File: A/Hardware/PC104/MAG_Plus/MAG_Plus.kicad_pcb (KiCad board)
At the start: 2 copper layers, 96 x 89.9 mm, 106 parts, among them J1 RPi_GPIO, J2 U.FL-R-SMT(01), J3 U.FL-R-SMT(01), J4 U.FL-R-SMT(01), J5 U.FL-R-SMT(01), J6 Conn_01x12_Male, J7 Conn_01x04_Male, J8 Conn_01x04_Male, J9 Conn_01x06_Male, SW1 SW_Push, U1 Payload, U10 QPQ1906SR, U11 ISO7341C, U12 PIC16F1847-I_SO, U13 LP38693MP-3.3, U14 LP38693MP-3.3, U15 LP38693MP-5.0, U16 LP38693MP-3.3, U2 ISO1540, U3 ISO7341C, U4 AD8302, U5 AD8302, U6 AD7904BRUZ-REEL7, U7 QPQ1906SR, U8 QPQ1906SR, U9 QPQ1906SR

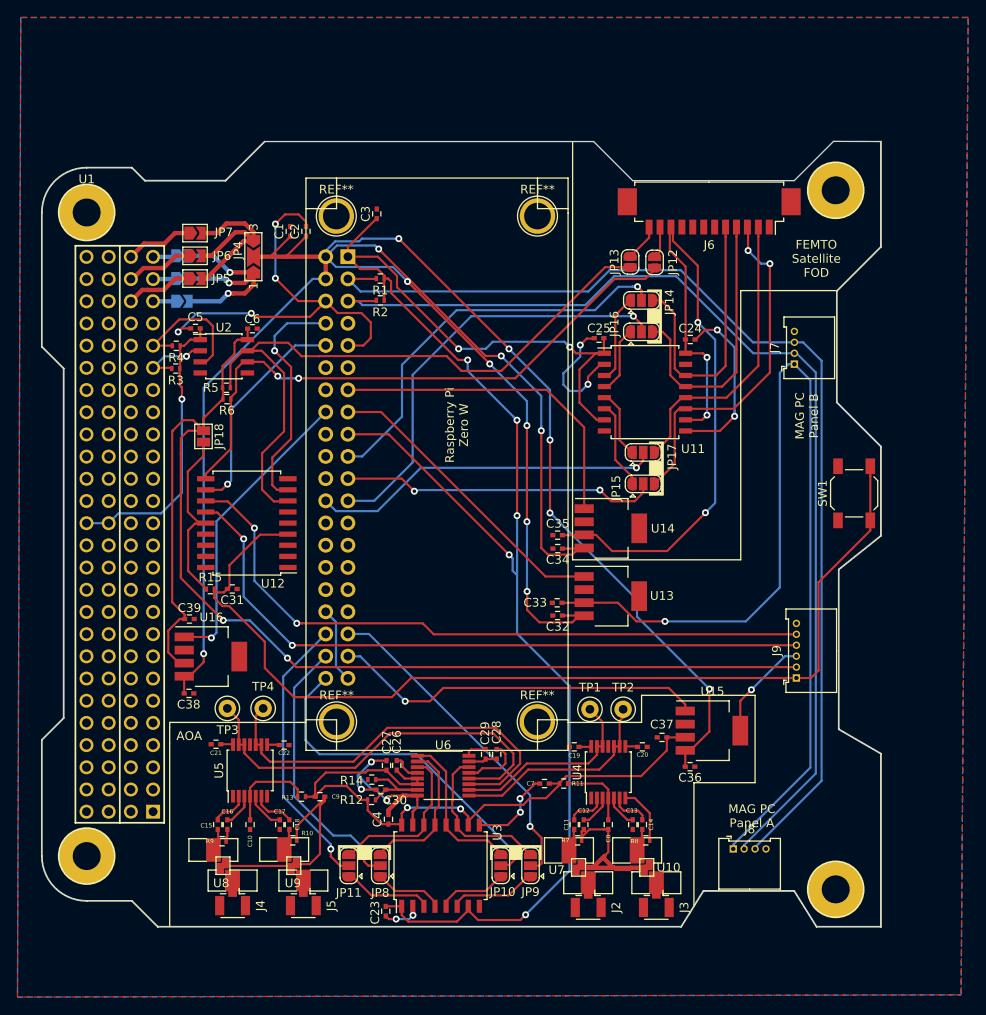
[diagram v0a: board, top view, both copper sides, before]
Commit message: new modifications pcb
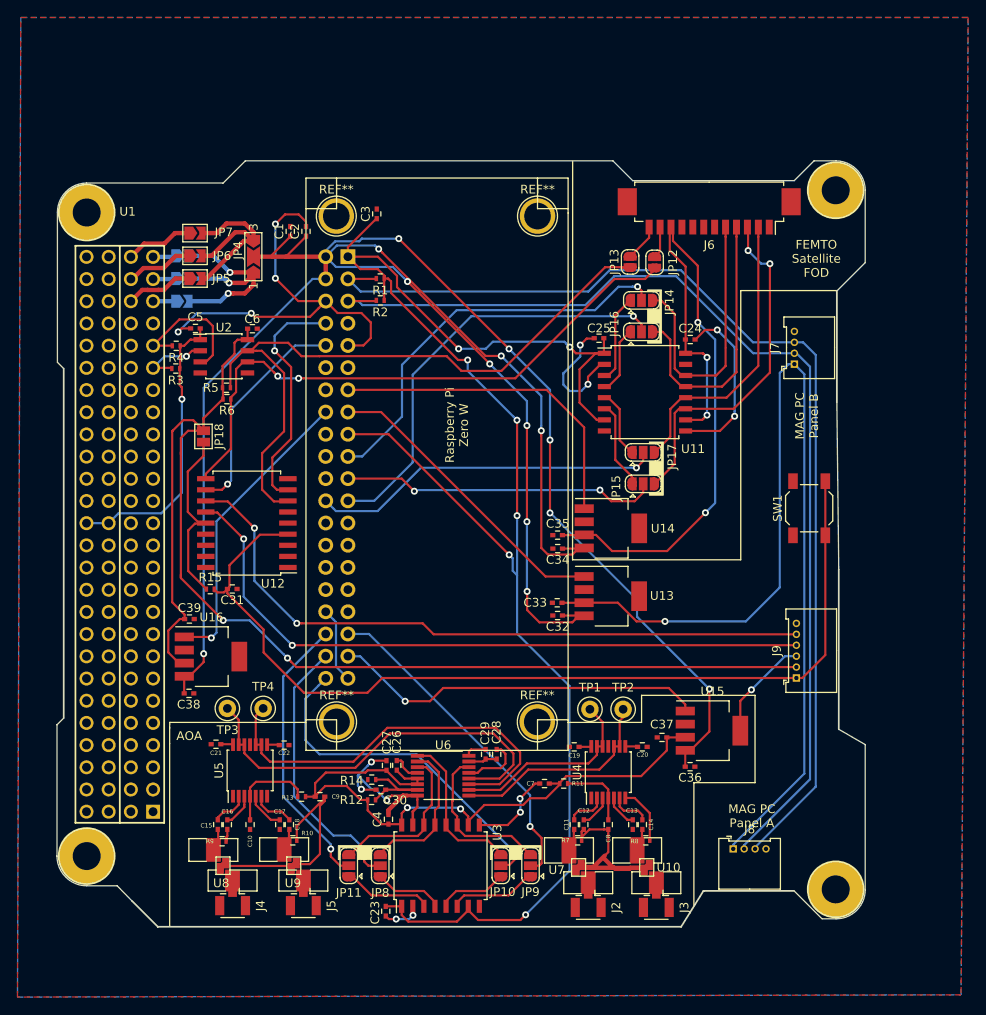
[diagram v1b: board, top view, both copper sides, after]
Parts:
- moved SW1 5.43 mm to (193.2, 94.6)
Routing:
- net MCLR: track 116.4 -> 109.5 mm
- net MAG_3V3: track 113.9 -> 113.3 mm
- net RPI_SDA: track 122.3 -> 121.8 mm
- net RPI_SCL: track 120.8 -> 120.3 mm
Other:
- board size 96 x 89.9 mm -> 92.5 x 86.8 mm
